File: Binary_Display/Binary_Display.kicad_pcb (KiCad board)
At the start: 2 copper layers, 46 parts, among them U1 MAX_7219

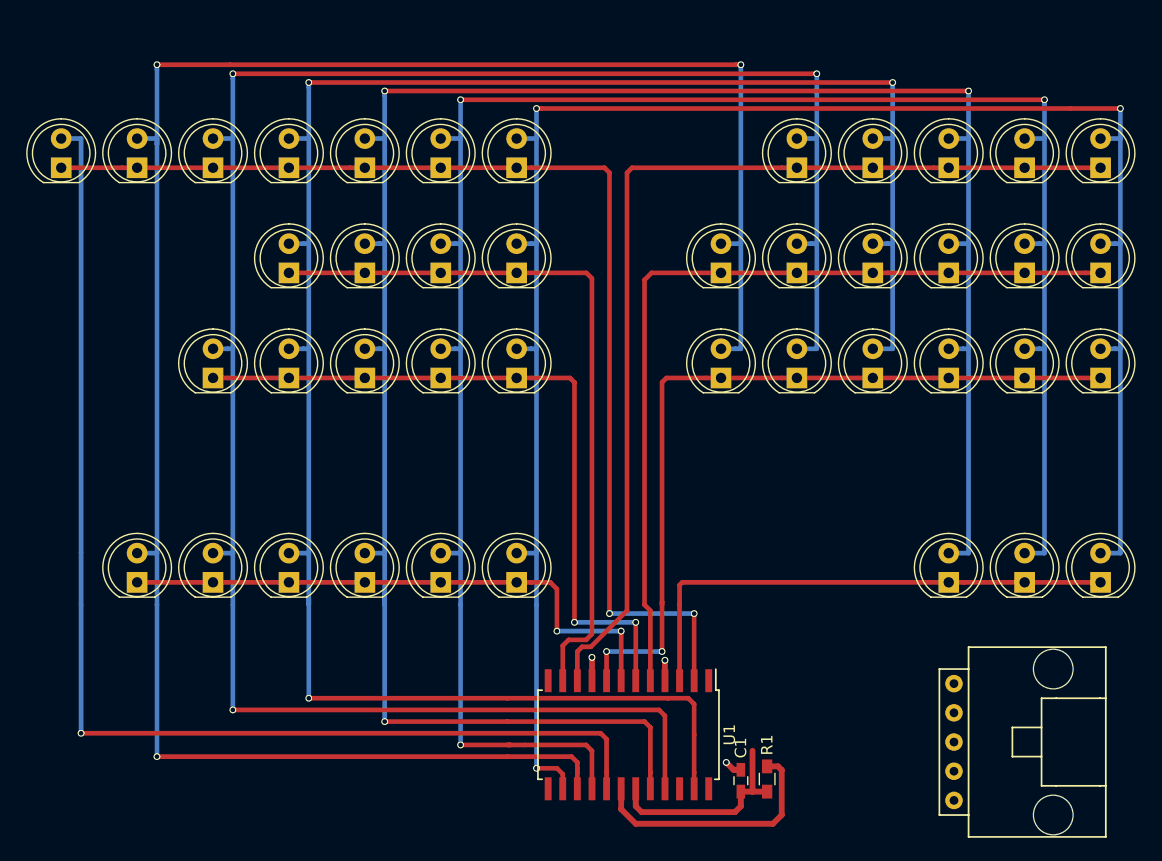
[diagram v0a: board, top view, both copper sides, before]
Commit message: Changes
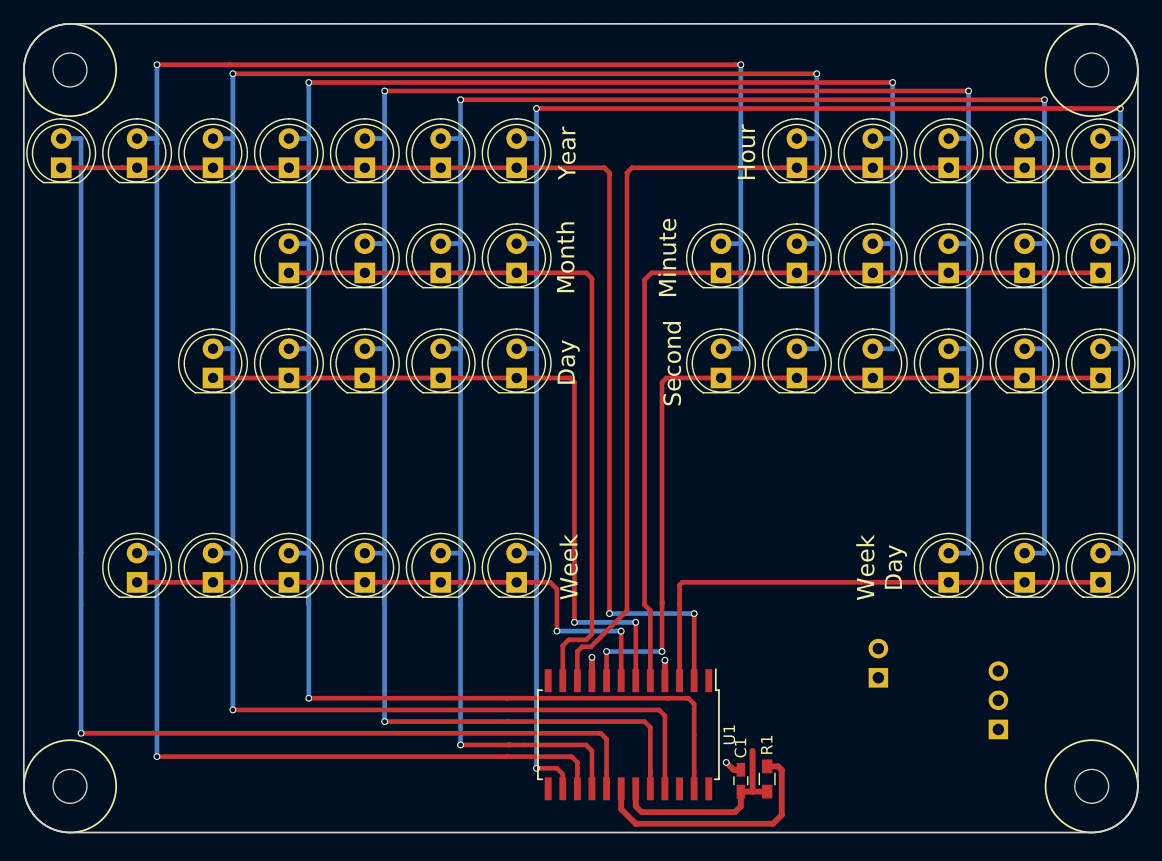
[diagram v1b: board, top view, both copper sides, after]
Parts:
- removed Conn1: Molex_SL_5, MRDT_Connectors:MOLEX_SL_5_Horizontal
- added J1: Conn_01x02, Socket_Strips:Socket_Strip_Straight_1x02_Pitch2.54mm, B.Cu at (191.0, 130.8)
- added J2: Conn_01x03, Socket_Strips:Socket_Strip_Straight_1x03_Pitch2.54mm, B.Cu at (201.5, 135.3)
- added REF**: 4_40_Hole, MRDT_Drill_Holes:4_40_Hole_Corner, F.Cu at (205.6, 81.9)
- added REF**: 4_40_Hole, MRDT_Drill_Holes:4_40_Hole_Corner, F.Cu at (124.7, 136.2)
- added REF**: 4_40_Hole, MRDT_Drill_Holes:4_40_Hole_Corner, F.Cu at (205.6, 136.2)
- added REF**: 4_40_Hole, MRDT_Drill_Holes:4_40_Hole_Corner, F.Cu at (124.7, 81.9)
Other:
- board outline added: 96.9 x 70.4 mm
- board text added: "Day"
- board text added: "Hour"
- board text added: "Minute"
- board text added: "Month"
- board text added: "Second"
- board text added: "Week"
- board text added: "Week Day"
- board text added: "Year"
